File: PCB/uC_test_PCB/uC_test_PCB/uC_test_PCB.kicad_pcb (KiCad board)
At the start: 2 copper layers, 105.8 x 15 mm, 35 parts, among them J1 781710004, J3 SM03B-SRSS-TB, J4 SM03B-SRSS-TB, Q3 DMG2305, SW101 KMR2, SW102 KMR2, U1 Core52840, U2 AP2112(3.3V), U3 MCP73831T-2ACI/OT, X3 JSTPH

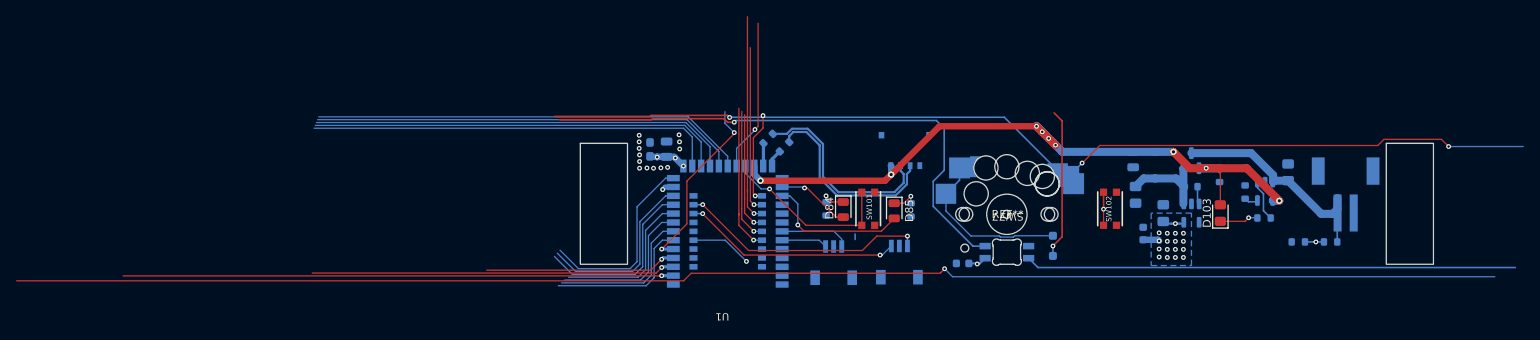
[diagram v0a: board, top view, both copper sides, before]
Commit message: small changes to test pcb
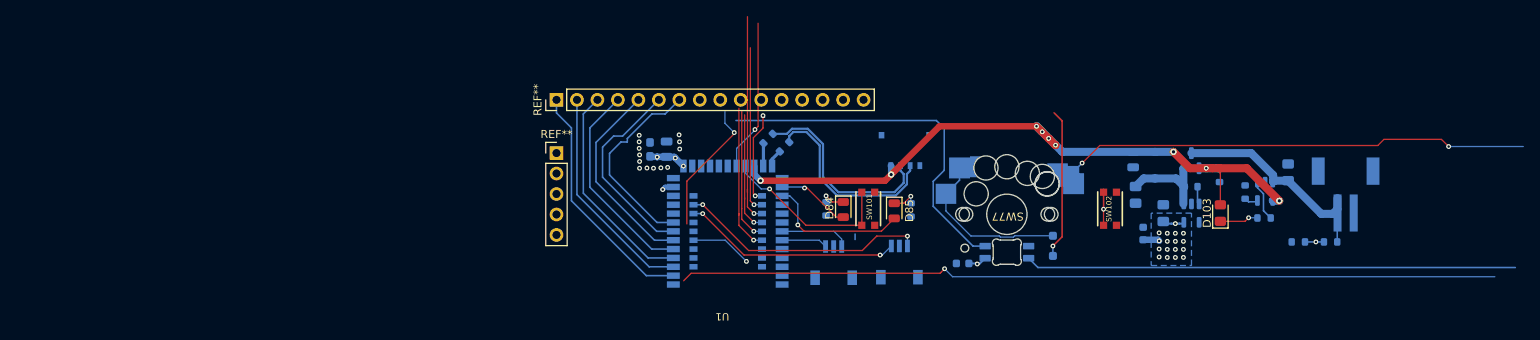
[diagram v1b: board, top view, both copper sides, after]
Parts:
- removed the REF** at (160.2, 118.3)
- added REF**: PinHeader_1x16_P2.54mm_Vertical, Connector_PinHeader_2.54mm:PinHeader_1x16_P2.54mm_Vertical, F.Cu at (104.3, 104.1)
- added REF**: PinHeader_1x05_P2.54mm_Vertical, Connector_PinHeader_2.54mm:PinHeader_1x05_P2.54mm_Vertical, F.Cu at (104.3, 110.7)
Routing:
- net (no net): track 1521.5 -> 986.3 mm, vias 76 -> 70
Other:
- board size 105.8 x 15 mm -> 3.6 x 3.3 mm
